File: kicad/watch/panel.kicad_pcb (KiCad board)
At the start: 2 copper layers, 34.1 x 41.7 mm, 68 parts, among them IC1 113990582, IC2 M41T62LC6F, J1 Conn_01x04_Female, J1 USB_C_Receptacle_USB2.0, J2 Conn_01x04_Female, J3 Buzzer, J4 Memory LCD, J5 Conn_01x04_Female, P1 AXT510124, P1 AXT610124, Q1 DMN6140L, Q2 DMN6140L, U1 MAX17260, U1 W25X20CLUXIG, U2 MCP73831-2-OT, U3 TPS63001, U4 TPS61222DCK, Y1 Crystal

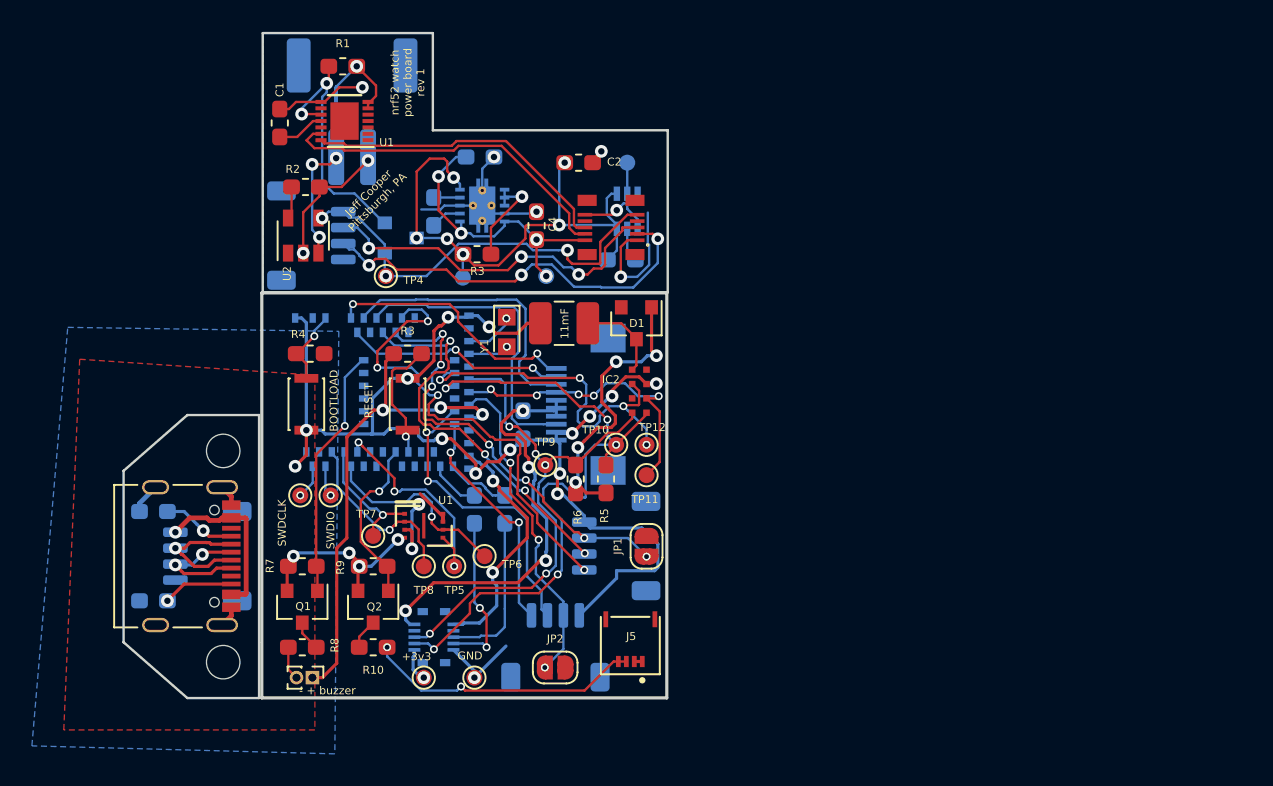
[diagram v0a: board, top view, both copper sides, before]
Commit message: snapshot for upload to github, now that copyrights are cleared
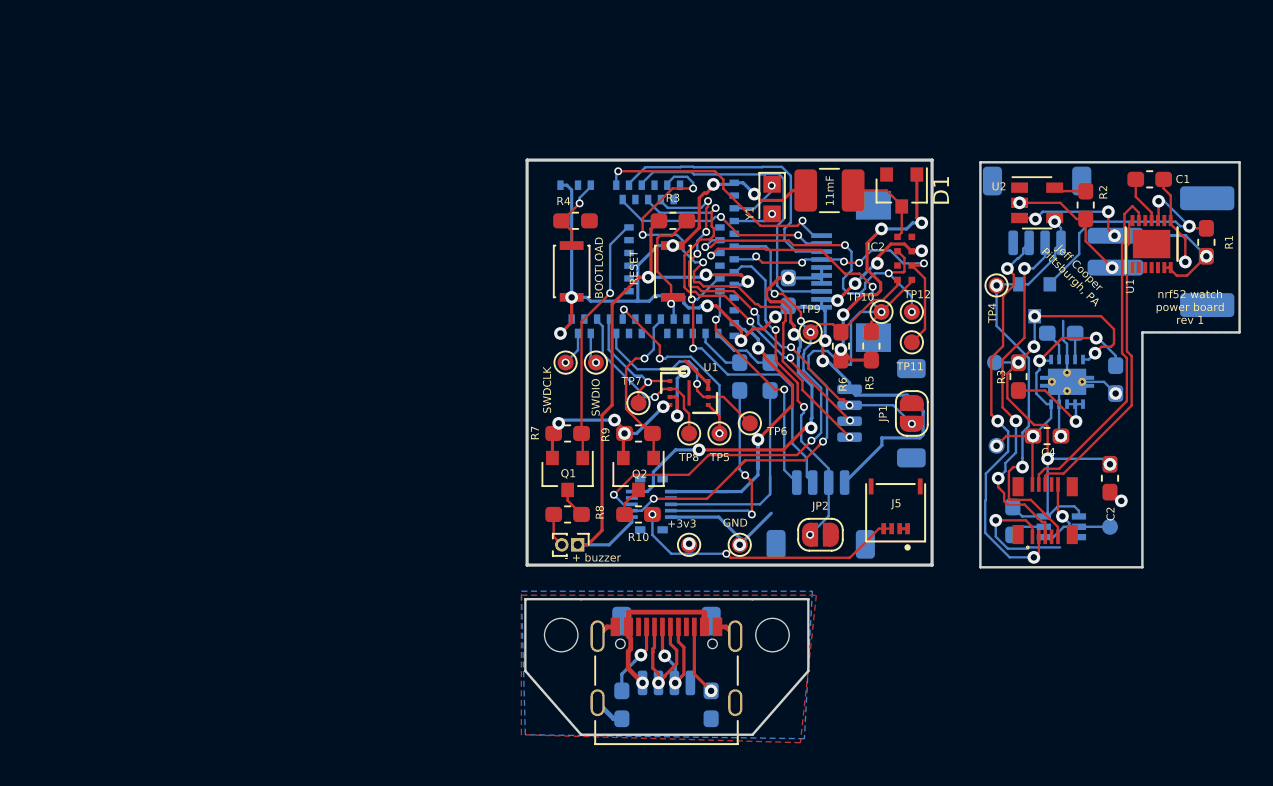
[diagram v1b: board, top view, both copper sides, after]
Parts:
- removed the REF** at (12.8, 42.8)
- removed the REF** at (12.8, 56.0)
- added REF**: MountingHole_2.1mm, MountingHole:MountingHole_2.1mm, F.Cu at (34.0, 54.3)
- added REF**: MountingHole_2.1mm, MountingHole:MountingHole_2.1mm, F.Cu at (47.2, 54.3)
- moved R1 55.3 mm to (74.4, 29.7), turned to 270 degrees
- moved C1 54.7 mm to (70.9, 25.7), turned to 0 degrees
- moved BT1 51.5 mm to (71.6, 30.3), turned to 270 degrees
- moved U1 51.2 mm to (71.0, 29.8), turned to 90 degrees
- moved R2 48.9 mm to (66.8, 27.3), turned to 270 degrees
- moved U2 46.1 mm to (63.8, 27.2), turned to 0 degrees
- moved J1 45.5 mm to (63.8, 27.7), turned to 0 degrees
- moved C3 42.2 mm to (68.7, 38.3), turned to 270 degrees
- moved L1 40.1 mm to (65.3, 35.4), turned to 180 degrees
- moved D1 40.0 mm to (63.6, 33.3), turned to 270 degrees
- moved C2 38.8 mm to (68.4, 44.5), turned to 270 degrees
- moved TP4 38.3 mm to (61.3, 32.4), turned to 270 degrees
- moved U3 38.3 mm to (65.7, 38.4), turned to 270 degrees
- moved TP3 37.9 mm to (68.4, 47.5), turned to 270 degrees
- moved R2 35.6 mm to (43.4, 58.7), turned to 90 degrees
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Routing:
- net SCL: track 55.6 -> 61.2 mm
- net VBUS: track 52.5 -> 57.6 mm
- net USB_DN: track 32.6 -> 36.8 mm
- net SDA: track 65.3 -> 69.1 mm
- net USB_DP: track 35.9 -> 39.5 mm
- net GND: track 130.6 -> 133.6 mm
- net +5V: track 33.6 -> 36.1 mm
- net +3V3: track 77.1 -> 79.4 mm
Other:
- board size 34.1 x 41.7 mm -> 44.8 x 36 mm
- net class Default: clearance 0.2 -> 0.15; trace_width 0.2 -> 0.15
- net class pow removed
- rule trace_clearance: 0.2 -> 0.15
- rule trace_min: 0.2 -> 0.1
- rule via_min_size: 0.4 -> 0.2
